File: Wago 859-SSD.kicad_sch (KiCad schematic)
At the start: 17 parts, among them J1 IN+, J2 IN-, J3 OUT VB, J5 OUT+, J8 OUT1-, Q2 BSS138, Q3 BSS84, U1 PC817

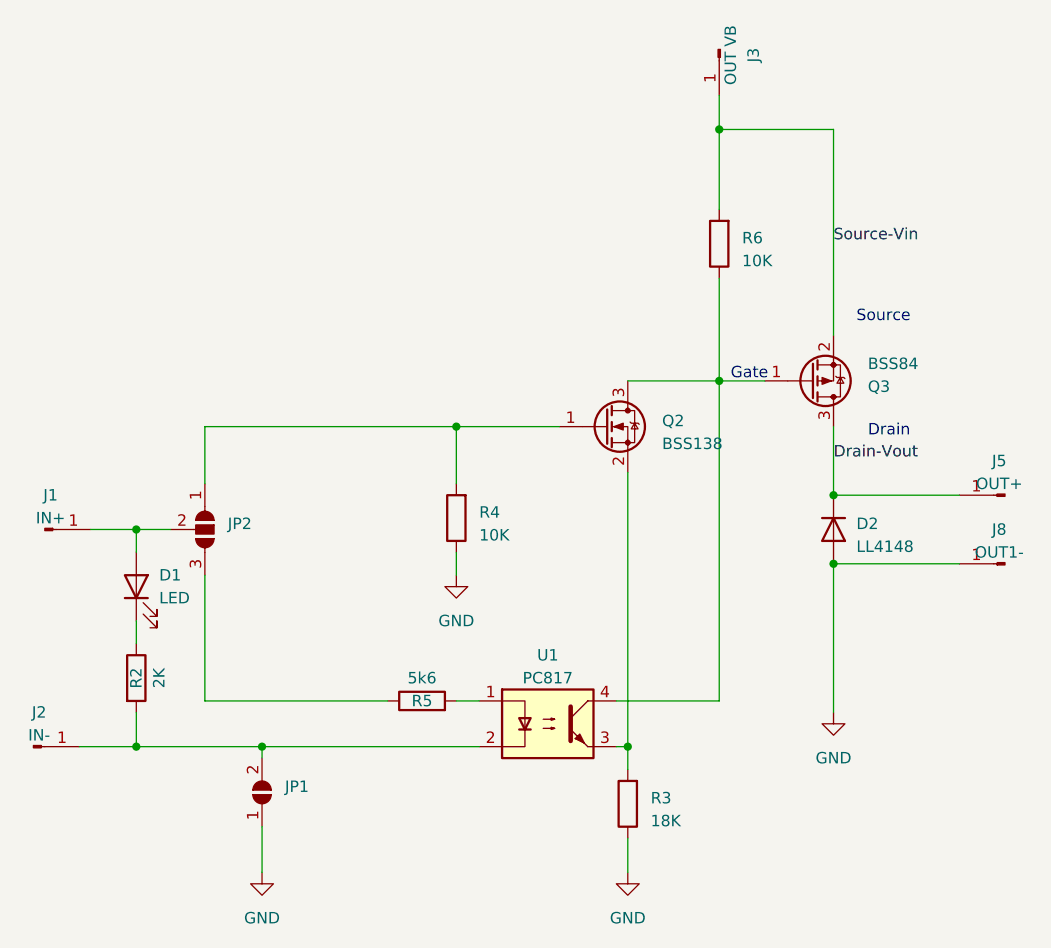
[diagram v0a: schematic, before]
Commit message: Bugfix Version: V3
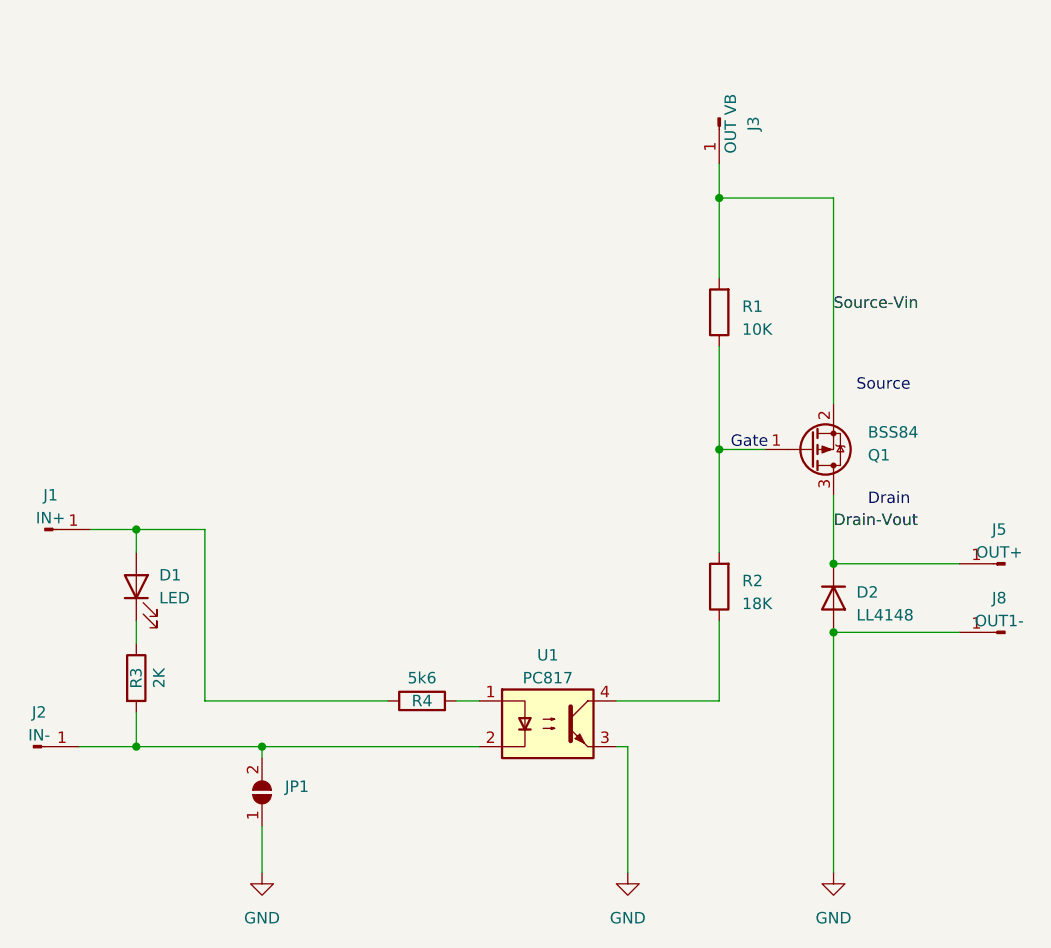
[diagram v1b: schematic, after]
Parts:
- removed JP2: SolderJumper_3_Open, Jumper:SolderJumper-3_P1.3mm_Open_Pad1.0x1.5mm, symbol Jumper:SolderJumper_3_Open
- removed Q2: BSS138, Package_TO_SOT_SMD:SOT-23_Handsoldering, symbol Transistor_FET:BSS138
- removed R4: 10K, Resistor_SMD:R_0805_2012Metric_Pad1.20x1.40mm_HandSolder, symbol Device:R
- renumbered Q3 to Q1, R6 to R1, R3 to R2, R2 to R3, R5 to R4
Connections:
- net GND: now also U1.3; no longer R2.1
- net at R2.2: now also Q1.1 (G), R1.1; no longer U1.3
- net at D1.2 (A), J1.1 (Pin_1): now also R4.1
- new net: R2.1, U1.4
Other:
- moved on the sheet: D2, J3, J5, J8, Q1, R1, R2
